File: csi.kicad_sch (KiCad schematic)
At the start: 69 parts, among them J1 522071560, J12 522071560, J6 522071560, J9 522071560, U24 AP22615A, U25 AP22615A, U26 PI4MSD5V9548AZDEX, U3 AP22615A, U31 NTS0102, U32 NTS0102, U7 AP22615A

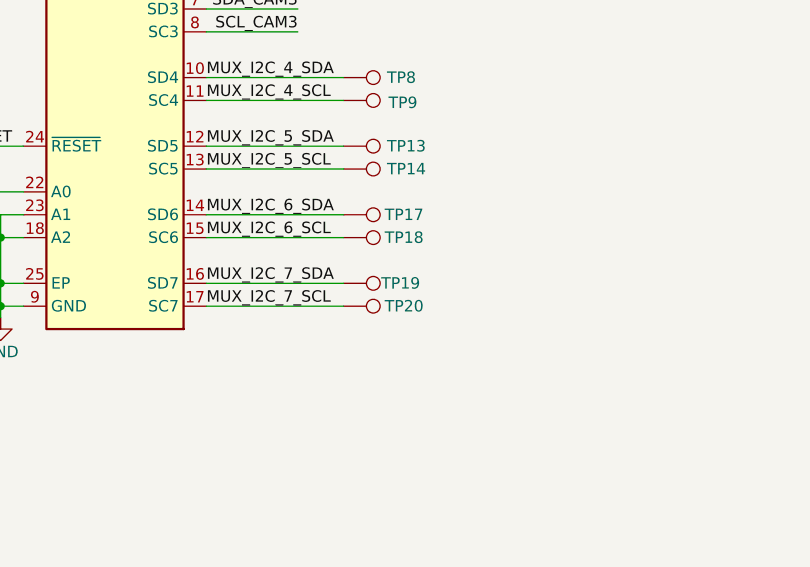
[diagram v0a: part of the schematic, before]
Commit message: v2.1 Updates
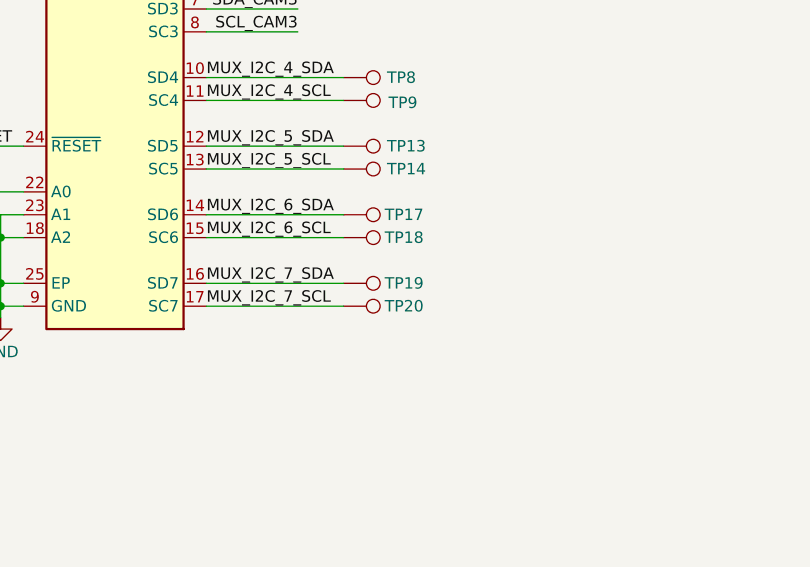
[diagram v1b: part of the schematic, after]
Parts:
- C100, C101, C39, C43, C47, C79, C89, C96, C97: Author Antmicro -> (none); Dielectric X5R -> (none); License Apache-2.0 -> (none); MPN GRM155R61H104KE14D -> C307348; Val 100n -> (none); Voltage 50V -> (none)
- D10, D11, D12, D13: Author Antmicro -> (none); License Apache-2.0 -> (none); MPN LTST-C190GKT -> C2909774; Manufacturer Lite-On -> (none); Public False -> (none)
- R10, R2, R51, R6: Author Antmicro -> (none); License Apache-2.0 -> (none); MPN CR0402-FX-1003GLF -> C237792; Manufacturer Bourns -> (none); Tolerance 1% -> (none); Val 100k -> (none)
- R101, R102, R26, R36, R48, R54, R55, R63: MPN (none) -> C2076947
- R142, R35, R53: Author Antmicro -> (none); Current 1A -> (none); License Apache-2.0 -> (none); MPN ERJ2GE0R00X -> C190119; Manufacturer Panasonic -> (none); Val 0R -> (none)
- R144, R3, R64, R66, R67: Author Antmicro -> (none); License Apache-2.0 -> (none); MPN CR0402-FX-1002GLF -> C2479067; Manufacturer Bourns -> (none); Tolerance 1% -> (none); Val 10k -> (none)
- R180, R182, R183, R184, R185, R34, R40, R50, R9, TP13, TP14, TP17, TP18, TP19, TP20, TP8, TP9: now left out of the parts list
- R7, R8, R85, R86, R87, R88, R89, R90: Author Antmicro -> (none); License Apache-2.0 -> (none); MPN CR0402-FX-4701GLF -> C844931; Manufacturer Bourns -> (none); Tolerance 1% -> (none); Val 4k7 -> (none)
- U24, U25, U3, U7: Author Antmicro -> (none); License Apache-2.0 -> (none); MPN AP22615AWU-7 -> C2680357; Manufacturer Diodes Incorporated -> (none)
